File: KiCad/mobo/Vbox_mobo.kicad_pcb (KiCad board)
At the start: 2 copper layers, 172 x 107 mm, 56 parts, among them J1 Conn_01x02, J2 JTAG_TC2030, J3 DuPont Connector, SW1 Boot, U1 XC6206, U2 X05A26H12G, U3 RP2040, U4 W25Q128JVS, Y1 12MHz

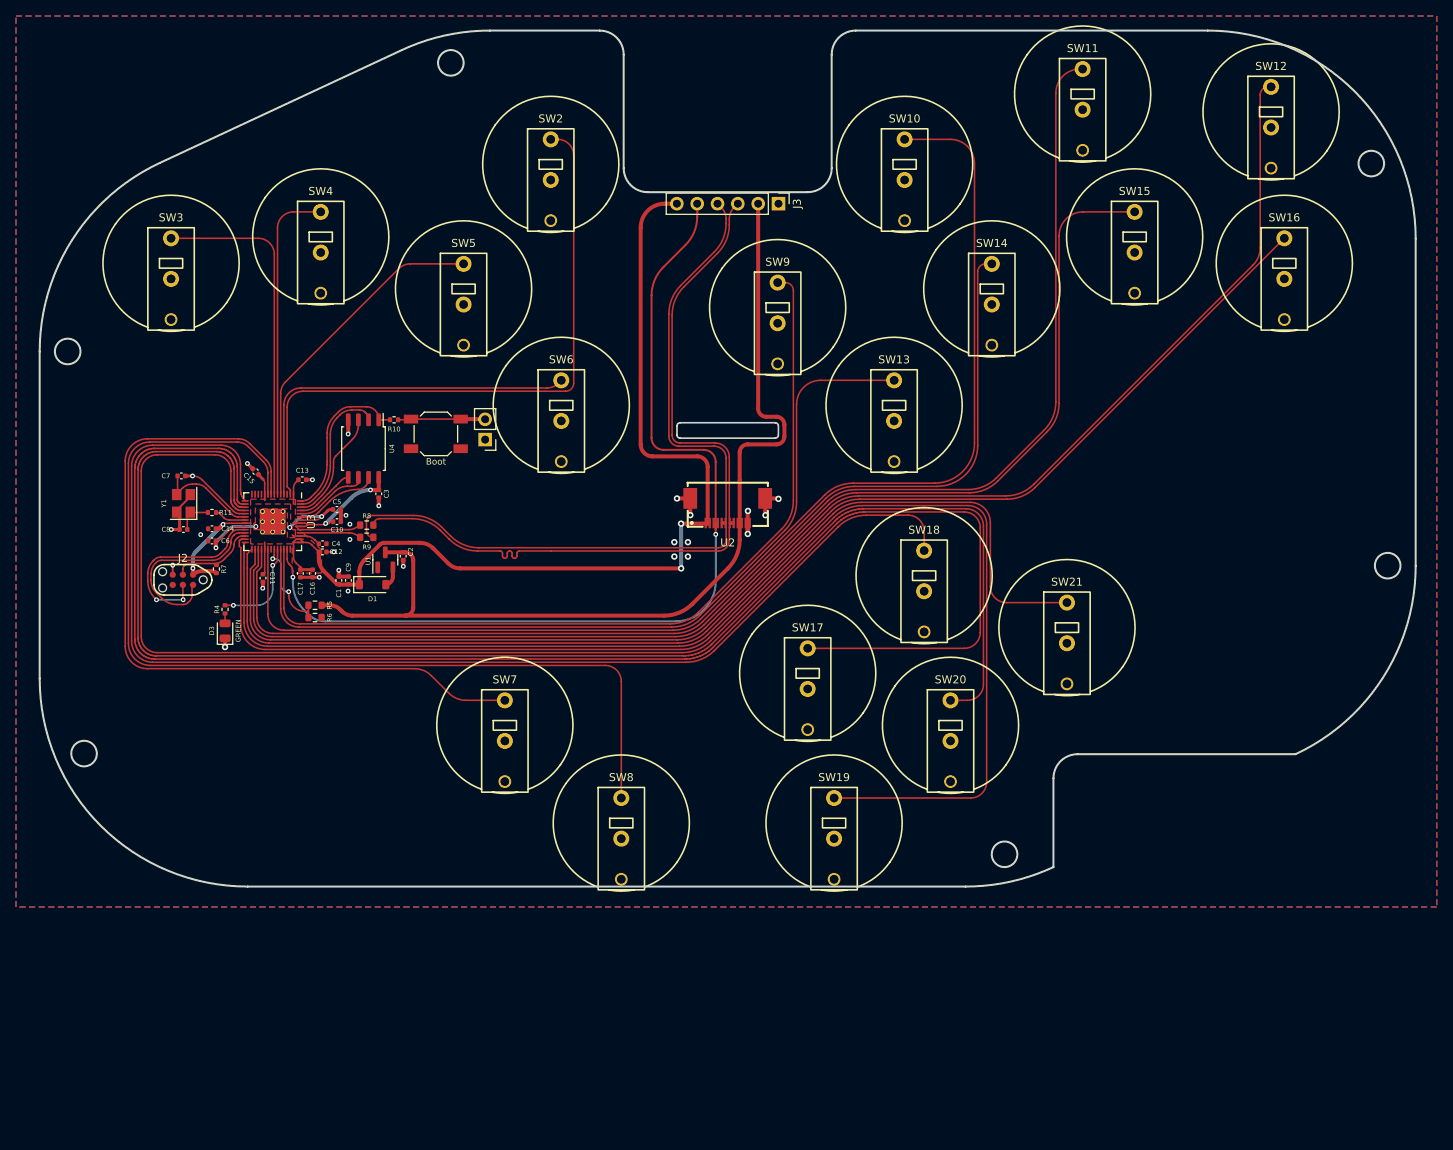
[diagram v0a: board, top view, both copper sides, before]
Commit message: mobo complete...?
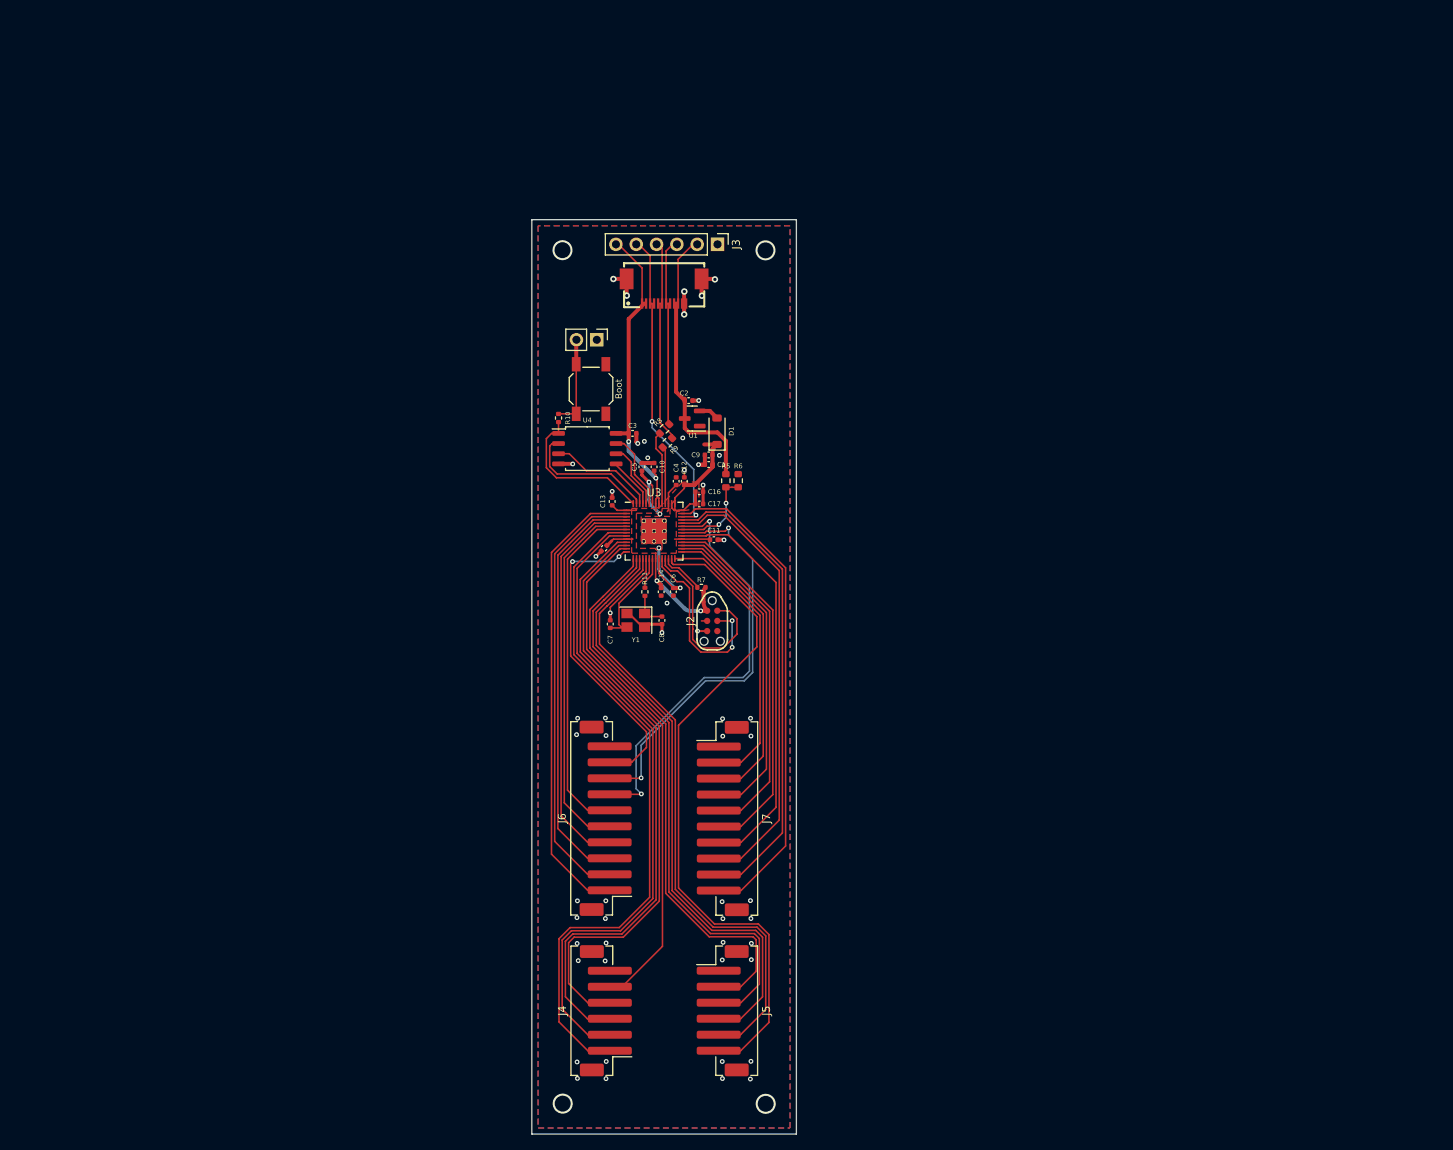
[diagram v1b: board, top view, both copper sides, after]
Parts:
- removed D3: GREEN, LED_SMD:LED_0805_2012Metric
- removed R4: 470, Resistor_SMD:R_0402_1005Metric
- removed SW10, SW11, SW12, SW13, SW14, SW15, SW16, SW17, SW18, SW19, SW2, SW20, SW21, SW3, SW4, SW5, SW6, SW7, SW8, SW9: ~, Buttons:RanaTadpole
- added J4: Conn_01x06, Connector_JST:JST_PH_B6B-PH-SM4-TB_1x06-1MP_P2.00mm_Vertical, F.Cu at (94.3, 140.8)
- added J5: Conn_01x06, Connector_JST:JST_PH_B6B-PH-SM4-TB_1x06-1MP_P2.00mm_Vertical, F.Cu at (108.9, 140.8)
- added J6: Conn_01x10, Connector_JST:JST_PH_B10B-PH-SM4-TB_1x10-1MP_P2.00mm_Vertical, F.Cu at (94.3, 116.7)
- added J7: Conn_01x10, Connector_JST:JST_PH_B10B-PH-SM4-TB_1x10-1MP_P2.00mm_Vertical, F.Cu at (108.9, 116.8)
- moved J2 66.4 mm to (107.6, 92.1), turned to -90 degrees
- moved C8 60.9 mm to (101.3, 92.0), turned to 90 degrees
- moved R7 60.7 mm to (106.3, 87.9), turned to 180 degrees
- moved Y1 58.4 mm to (98.1, 92.0), turned to 180 degrees
- moved C6 58.0 mm to (102.8, 88.4), turned to -90 degrees
- moved C7 56.7 mm to (94.9, 92.5), turned to -90 degrees
- moved C14 56.7 mm to (101.2, 88.4), turned to -90 degrees
- moved C11 56.6 mm to (107.8, 81.9), turned to 0 degrees
- moved R6 55.6 mm to (110.9, 74.5), turned to 90 degrees
- moved R11 55.0 mm to (99.2, 88.4), turned to 90 degrees
- moved R5 53.7 mm to (109.3, 74.5), turned to -90 degrees
- moved C17 50.6 mm to (106.0, 77.4), turned to 0 degrees
- moved C16 49.4 mm to (106.0, 75.9), turned to 0 degrees
- moved C1 48.4 mm to (107.2, 72.5), turned to 0 degrees
- moved U3 47.7 mm to (100.3, 80.8), turned to 0 degrees
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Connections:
- U3 pad 11: unconnected-(U3-GPIO8-Pad11) -> M3
- U3 pad 12: unconnected-(U3-GPIO9-Pad12) -> M4
- U3 pad 13: unconnected-(U3-GPIO10-Pad13) -> M5
- U3 pad 14: unconnected-(U3-GPIO11-Pad14) -> INDEX2
- U3 pad 3: unconnected-(U3-GPIO1-Pad3) -> UP2
- U3 pad 35: unconnected-(U3-GPIO23-Pad35) -> RING2
- U3 pad 37: PICO_LED -> PINKY2
- U3 pad 41: unconnected-(U3-GPIO29/ADC3-Pad41) -> RIGHTSTART
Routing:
- net MS: track 178.7 -> 37.9 mm
- net C_DN: track 207.7 -> 77.6 mm
- net UP: track 162.1 -> 35.8 mm
- net LS: track 166.3 -> 43.6 mm
- net C_LT: track 193.2 -> 73.3 mm
- net Z: track 155.9 -> 40.8 mm
- net A: track 181.5 -> 75.5 mm
- net Y: track 152.6 -> 51.4 mm
- net X: track 133.8 -> 46.4 mm
- net C_UP: track 153.9 -> 71.1 mm
- net +5V: track 117.8 -> 35.5 mm
- net DATA: track 119.1 -> 39.7 mm
- net M3: track 0.00 -> 78.8 mm
- net 3vDiode: track 164.8 -> 88.2 mm, vias 6 -> 4
- net D+: track 100.0 -> 24.0 mm
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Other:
- board size 172 x 107 mm -> 33.1 x 114.3 mm
